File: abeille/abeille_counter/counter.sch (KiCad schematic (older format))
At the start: 3 parts, among them IC1 ATMEGA328-P

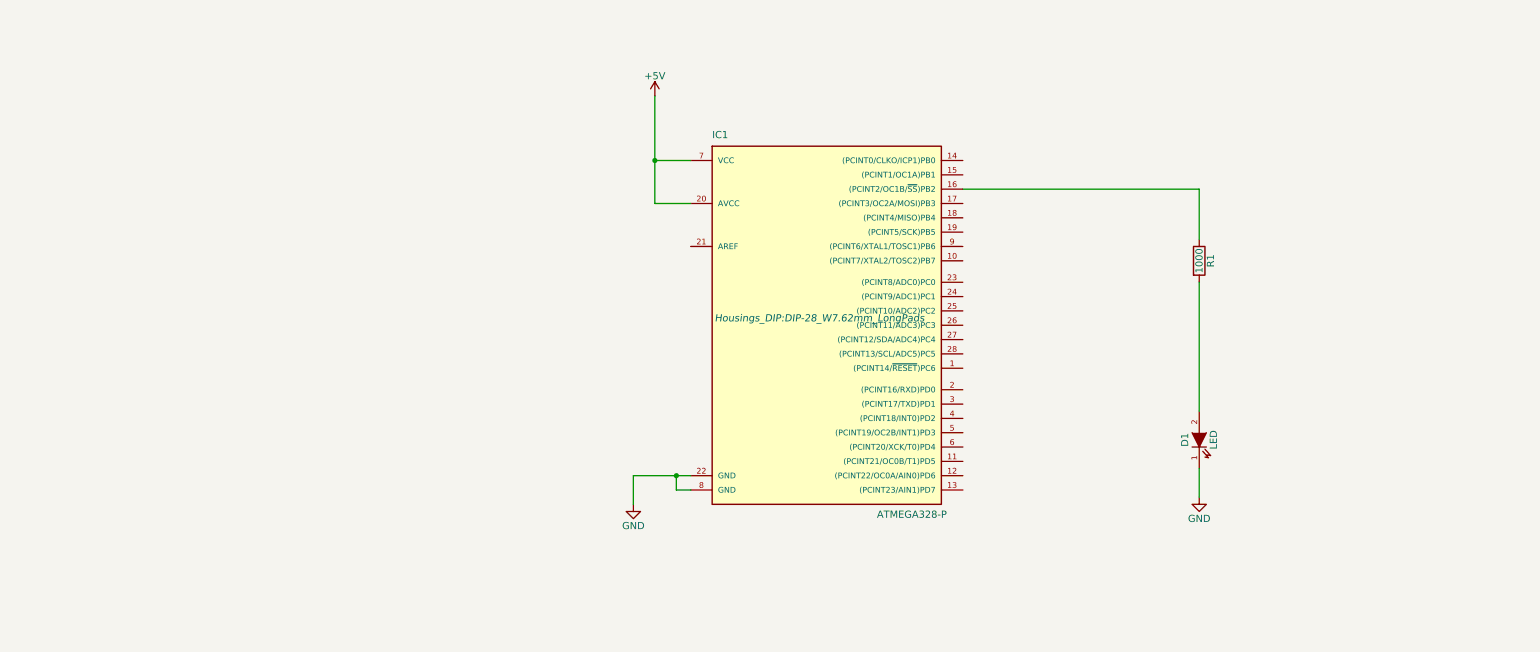
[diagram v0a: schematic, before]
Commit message: abeille counter schematics update
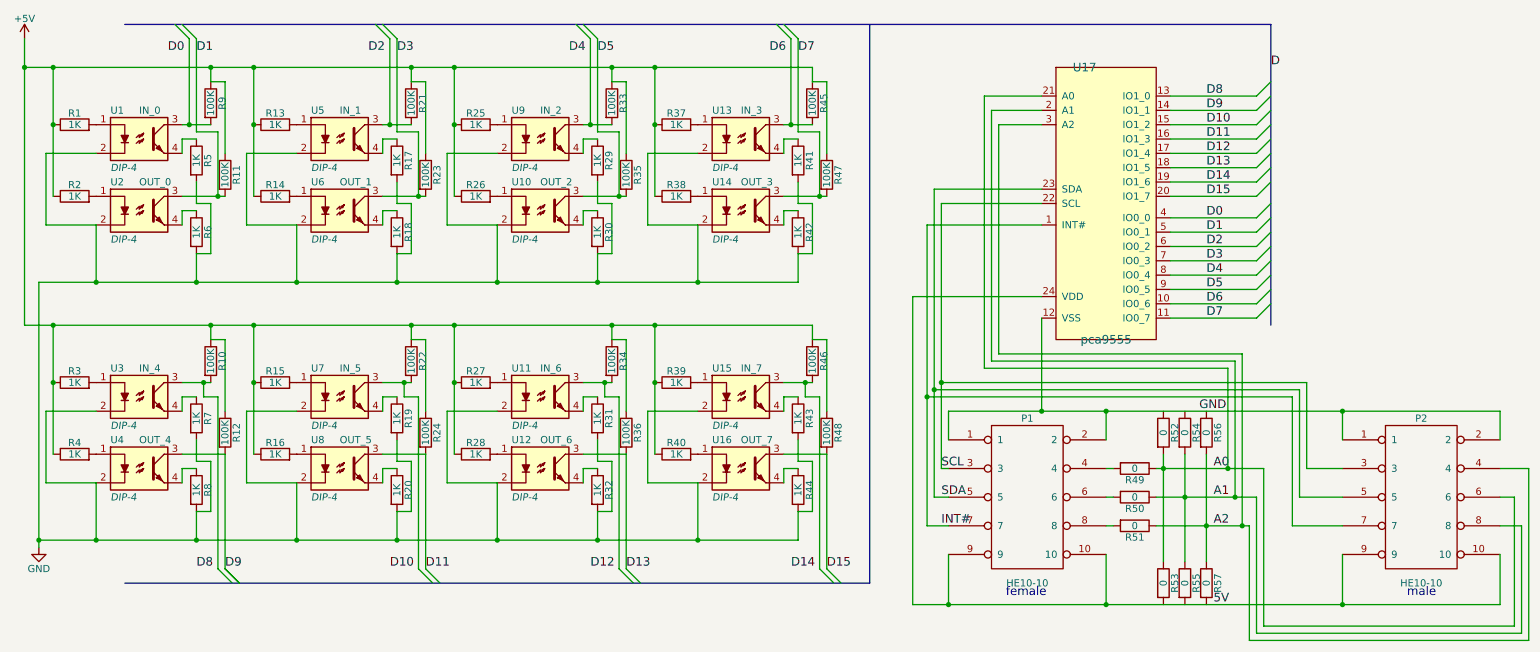
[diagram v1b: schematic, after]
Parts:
- removed D1: LED, LEDs:LED-3MM, symbol LED
- removed IC1: ATMEGA328-P, Housings_DIP:DIP-28_W7.62mm_LongPads, symbol ATMEGA328-P
- added P1, P2: HE10-10, symbol HE10-10
- added R10, R11, R12, R21, R22, R23, R24, R33, R34, R35, R36, R45, R46, R47, R48, R9: 100K, Resistors_ThroughHole:Resistor_Horizontal_RM10mm, symbol R
- added R13, R14, R15, R16, R17, R18, R19, R2, R20, R25, R26, R27, R28, R29, R3, R30, R31, R32, R37, R38, R39, R4, R40, R41, R42, R43, R44, R5, R6, R7, R8: 1K, Resistors_ThroughHole:Resistor_Horizontal_RM10mm, symbol R
- added R49, R50, R51, R52, R53, R54, R55, R56, R57: 0, Resistors_ThroughHole:Resistor_Horizontal_RM10mm, symbol R
- added U1: IN_0, DIP-4, symbol ITR-9608
- added U10: OUT_2, DIP-4, symbol ITR-9608
- added U11: IN_6, DIP-4, symbol ITR-9608
- added U12: OUT_6, DIP-4, symbol ITR-9608
- added U13: IN_3, DIP-4, symbol ITR-9608
- added U14: OUT_3, DIP-4, symbol ITR-9608
- added U15: IN_7, DIP-4, symbol ITR-9608
- added U16: OUT_7, DIP-4, symbol ITR-9608
- added U17: pca9555, symbol pca9555
- added U2: OUT_0, DIP-4, symbol ITR-9608
- added U3: IN_4, DIP-4, symbol ITR-9608
- added U4: OUT_4, DIP-4, symbol ITR-9608
- added U5: IN_1, DIP-4, symbol ITR-9608
- added U6: OUT_1, DIP-4, symbol ITR-9608
- added U7: IN_5, DIP-4, symbol ITR-9608
- added U8: OUT_5, DIP-4, symbol ITR-9608
- added U9: IN_2, DIP-4, symbol ITR-9608
- R1: value 1000 -> 1K
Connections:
- net +5V: now also R1.1, R10.1, R11.1, R12.1, R13.1, R14.1, R15.1, R16.1, R2.1, R21.1, R22.1, R23.1, R24.1, R25.1, R26.1, R27.1, R28.1, R3.1, R33.1, R34.1, R35.1, R36.1, R37.1, R38.1, R39.1, R4.1, R40.1, R45.1, R46.1, R47.1, R48.1, R9.1
- net GND: now also P1.1, P1.2, P2.1, P2.2, R17.2, R18.2, R19.2, R20.2, R29.2, R30.2, R31.2, R32.2, R41.2, R42.2, R43.2, R44.2, R5.2, R6.2, R7.2, R8.2, U1.2, U10.2, U11.2, U12.2, U13.2, U14.2, U15.2, U16.2, U17.12 (VSS), U2.2, U3.2, U4.2, U5.2, U6.2, U7.2, U8.2, U9.2
- net at R1.2: now also U1.1
- new net: R9.2, U1.3
- new net: R5.1, U1.4
- new net: R2.2, U2.1
- new net: R6.1, U2.4
- new net: R13.2, U5.1
- new net: R21.2, U5.3
- new net: R17.1, U5.4
- new net: R14.2, U6.1
- new net: R18.1, U6.4
- new net: R25.2, U9.1
- new net: R33.2, U9.3
- new net: R29.1, U9.4
- new net: R26.2, U10.1
- new net: R30.1, U10.4
- new net: R37.2, U13.1
- new net: R45.2, U13.3
- new net: R41.1, U13.4
- new net: R38.2, U14.1
- new net: R42.1, U14.4
- new net: R3.2, U3.1
- new net: R10.2, U3.3
- new net: R7.1, U3.4
- new net: R4.2, U4.1
- new net: R8.1, U4.4
- new net: R15.2, U7.1
- new net: R22.2, U7.3
- new net: R19.1, U7.4
- new net: R16.2, U8.1
- new net: R20.1, U8.4
- new net: R27.2, U11.1
- new net: R34.2, U11.3
- new net: R31.1, U11.4
- new net: R28.2, U12.1
- new net: R32.1, U12.4
- new net: R39.2, U15.1
- new net: R46.2, U15.3
- new net: R43.1, U15.4
- new net: R40.2, U16.1
- new net: R44.1, U16.4
- new net: P1.4, R49.2
- new net: P1.6, R50.2
- new net: P1.8, R51.2
- new net 5V: P1.10, P1.9, P2.10, P2.9, U17.24 (VDD)
- new net A0: P2.6, R49.1, R52.2, R53.1, U17.21 (A0)
- new net A1: P2.8, R50.1, R54.2, R55.1, U17.2 (A1)
- new net A2: P2.4, R51.1, R56.2, R57.1, U17.3 (A2)
- new net D0: U17.4 (IO0_0)
- new net D1: R11.2, U17.5 (IO0_1), U2.3
- new net D10: U17.15 (IO1_2)
- new net D11: R24.2, U17.16 (IO1_3), U8.3
- new net D12: U17.17 (IO1_4)
- new net D13: R36.2, U12.3, U17.18 (IO1_5)
- new net D14: U17.19 (IO1_6)
- new net D15: R48.2, U16.3, U17.20 (IO1_7)
- new net D2: U17.6 (IO0_2)
- new net D3: R23.2, U17.7 (IO0_3), U6.3
- new net D4: U17.8 (IO0_4)
- new net D5: R35.2, U10.3, U17.9 (IO0_5)
- new net D6: U17.10 (IO0_6)
- new net D7: R47.2, U14.3, U17.11 (IO0_7)
- new net D8: U17.13 (IO1_0)
- new net D9: R12.2, U17.14 (IO1_1), U4.3
- new net INT#: P1.7, P2.7, U17.1 (INT#)
- new net SCL: P1.3, P2.3, U17.22 (SCL)
- new net SDA: P1.5, P2.5, U17.23 (SDA)
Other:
- note added: "female"
- note added: "male"
- moved on the sheet: R1
